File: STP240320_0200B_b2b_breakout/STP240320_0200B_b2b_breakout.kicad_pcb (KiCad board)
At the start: 2 copper layers, 35.6 x 59.2 mm, 18 parts, among them J1 Micro_SD_Card_Det_Hirose_DM3AT, J2 Conn_01x11, Q1 BSS138, U1 74HC4050D, U2 AP2112K-3.3, U3 LM809M3X-2.93

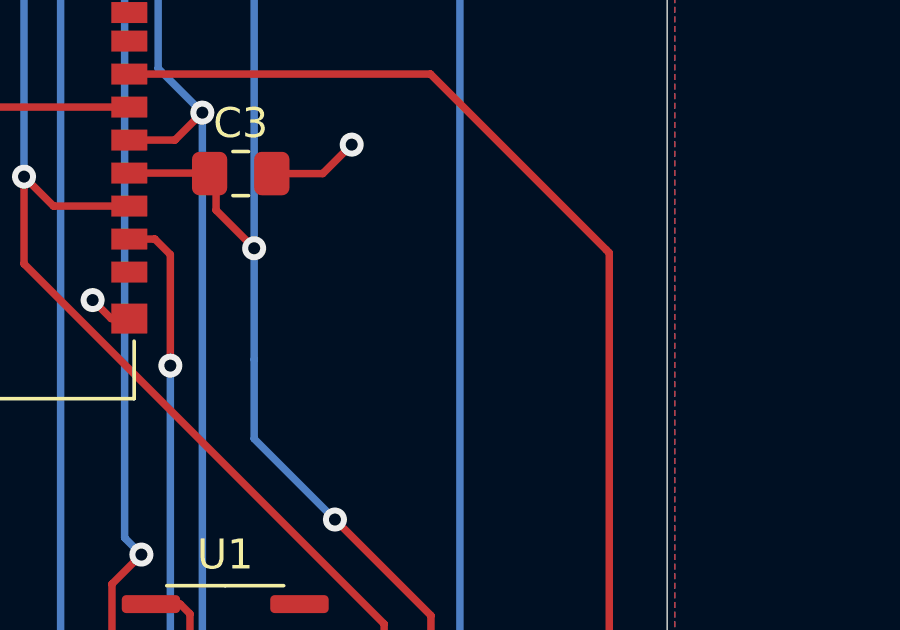
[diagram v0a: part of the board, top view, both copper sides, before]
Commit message: ci: add release support
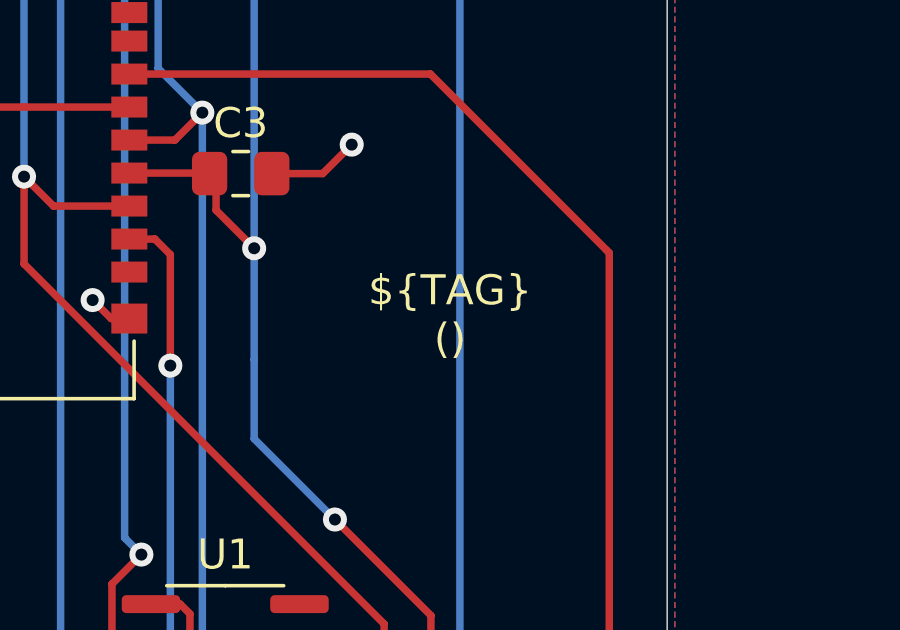
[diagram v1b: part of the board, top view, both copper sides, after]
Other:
- board text added: "${TAG} (${REVISION})"
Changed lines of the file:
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@@
     )
   )
+  (property "DATE" "YYYY-MM-DD HH:MM:SS")
+  (property "REVISION" "REVISION")
+  (property "TAG" "TAG")
   (net 0 "")
   (net 1 "Net-(DISP1-Pad2)")
@@
     (effects (font (size 1 1) (thickness 0.15)) (justify left))
   )
+  (gr_text "${TAG}\n(${REVISION})" (at 28.321 29.845) (layer "F.SilkS")
+    (effects (font (size 1 1) (thickness 0.15)))
+  )
   (segment (start 20.95 4.0844) (end 20.95 1.822) (width 0.25) (layer "F.Cu") (net 1))

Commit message: Revert "ci: add release support (#2)"
This reverts commit f3a1c30362bc760beaf5669eca90d55fbc6df8b2.
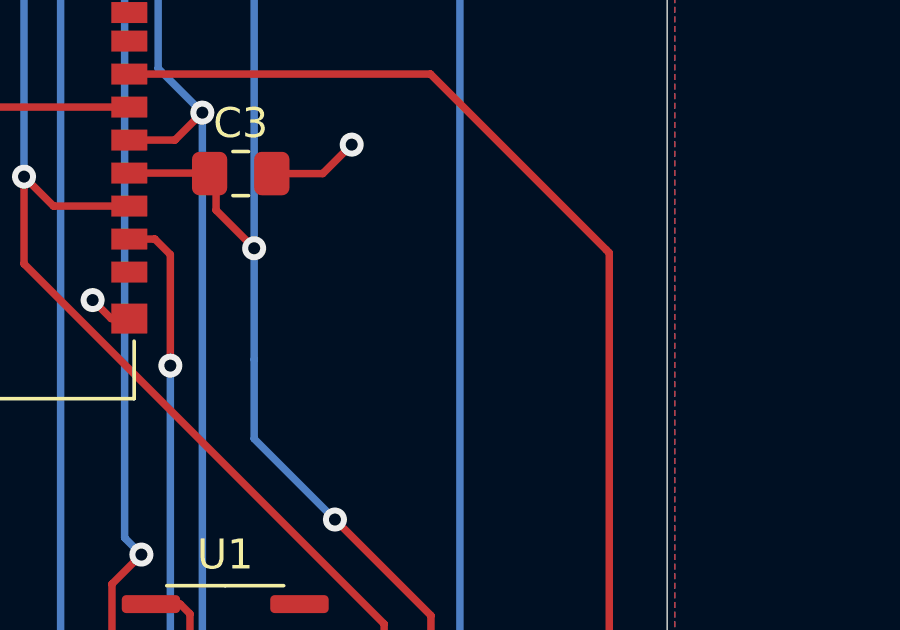
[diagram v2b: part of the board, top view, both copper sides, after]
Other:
- board text removed: "${TAG} (${REVISION})"
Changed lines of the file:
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@@
     )
   )
-  (property "DATE" "YYYY-MM-DD HH:MM:SS")
-  (property "REVISION" "REVISION")
-  (property "TAG" "TAG")
   (net 0 "")
   (net 1 "Net-(DISP1-Pad2)")
@@
     (effects (font (size 1 1) (thickness 0.15)) (justify left))
   )
-  (gr_text "${TAG}\n(${REVISION})" (at 28.321 29.845) (layer "F.SilkS")
-    (effects (font (size 1 1) (thickness 0.15)))
-  )
   (segment (start 20.95 4.0844) (end 20.95 1.822) (width 0.25) (layer "F.Cu") (net 1))
